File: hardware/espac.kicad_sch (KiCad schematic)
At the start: 67 parts, among them J1 USB_C_Receptacle_USB2.0_14P, J2 A3144, J3 A3144, J4 Conn_01x08, J5 Conn_01x10, J7 Conn_01x02, Q1 TEMT6000, SW1 RESET, SW2 BOOT, SW3 PRESS_PUSH, U1 ESP32-S3-WROOM-1, U2 AMS1117-3.3, U3 USBLC6-2SC6, U4 DS18B20, U5 SN74LVC1T45DBV

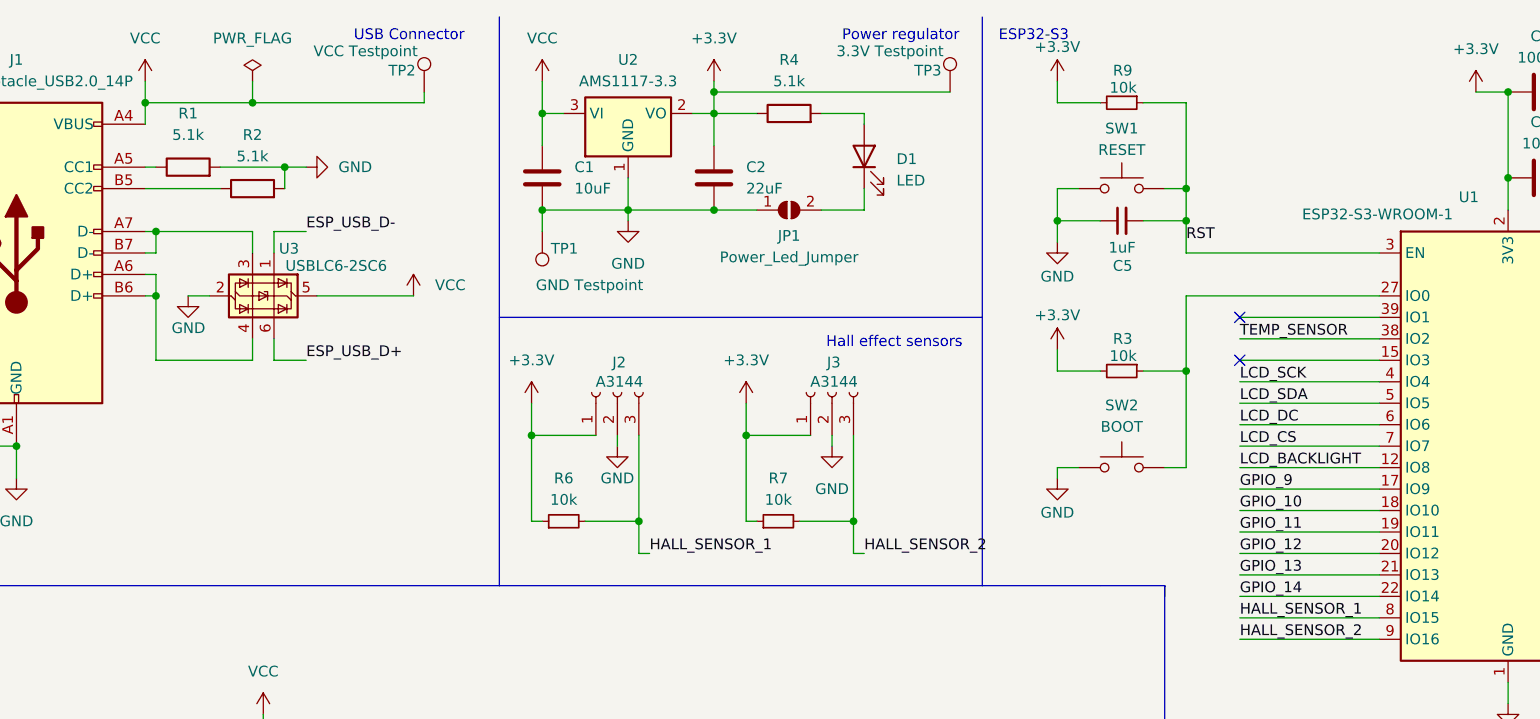
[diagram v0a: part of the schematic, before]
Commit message: pcb updates
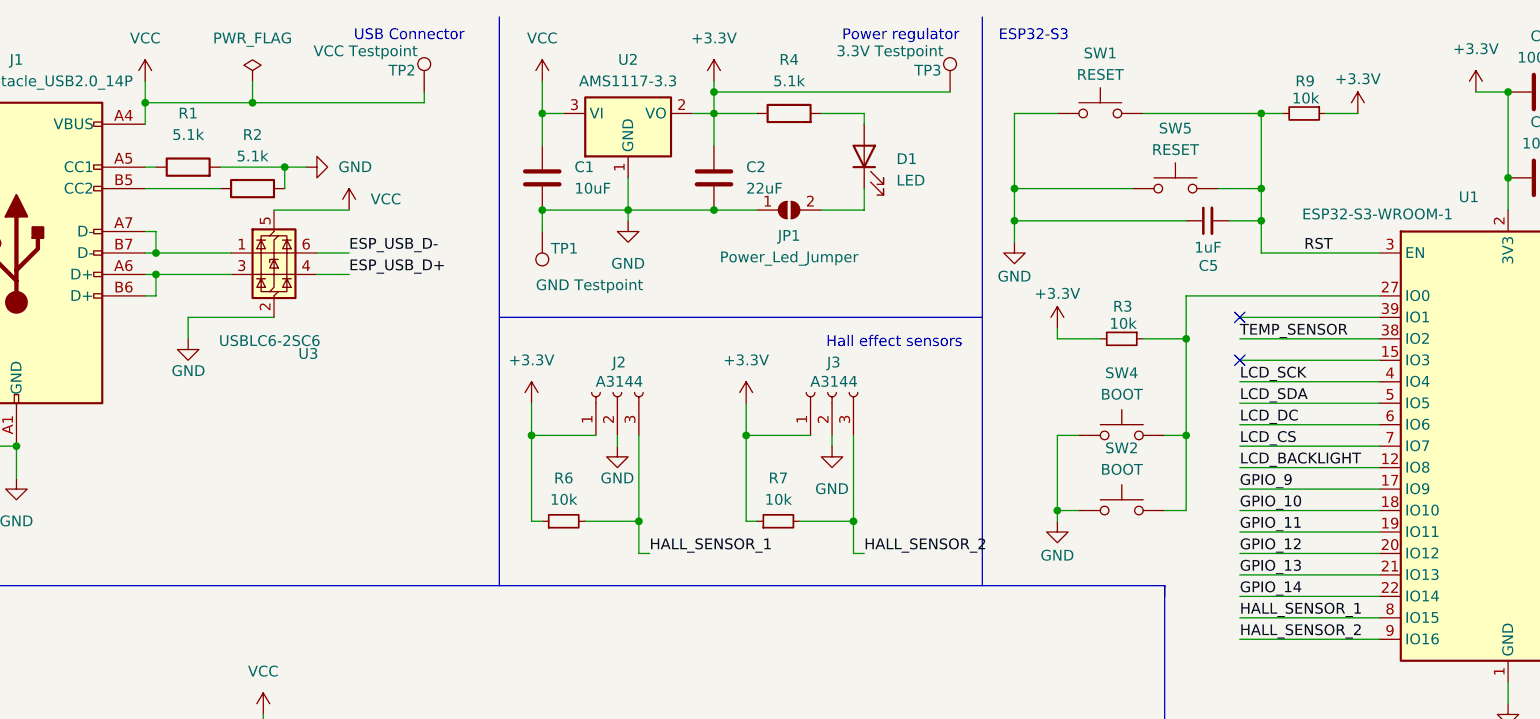
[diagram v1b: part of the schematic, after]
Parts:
- added SW4: BOOT, SMD_SIDED_TACT_SWITCH:SMD_TACT_SWITCH, symbol Switch:SW_Push
- added SW5: RESET, SMD_SIDED_TACT_SWITCH:SMD_TACT_SWITCH, symbol Switch:SW_Push
- SW1, SW2: footprint SW_TL3330AF130QG_EWI:SW_TL3330AF130QG_EWI -> SMD_SIDED_TACT_SWITCH:SMD_SIDED_TACT_SWITCH
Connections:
- net +3.3V: now also R9.1; no longer R9.2
- net ESP_USB_D+: now also U3.4 (I/O2); no longer U3.6 (I/O1)
- net ESP_USB_D-: now also U3.6 (I/O1); no longer U3.1 (I/O1)
- net GND: now also SW4.2, SW5.2
- net RST: now also R9.2, SW5.1; no longer R9.1
- net at R3.1, SW2.2, U1.27 (IO0): now also SW4.1
- net at J1.A6 (D+), J1.B6 (D+): now also U3.3 (I/O2); no longer U3.4 (I/O2)
- net at J1.A7 (D-), J1.B7 (D-): now also U3.1 (I/O1); no longer U3.3 (I/O2)
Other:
- moved on the sheet: C5, R3, R9, SW1, SW2, U3
